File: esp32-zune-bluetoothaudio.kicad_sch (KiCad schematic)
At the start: 36 parts, among them J1 Conn_01x06, J2 USB_C_Receptacle_USB2.0, J3 zune connector, Q1 MMBT3904, Q2 MMBT3904, Q3 MMBT3904, Q4 MMBT3904, U1 TPM, U2 ESP32-A1S, U3 AP1117-33

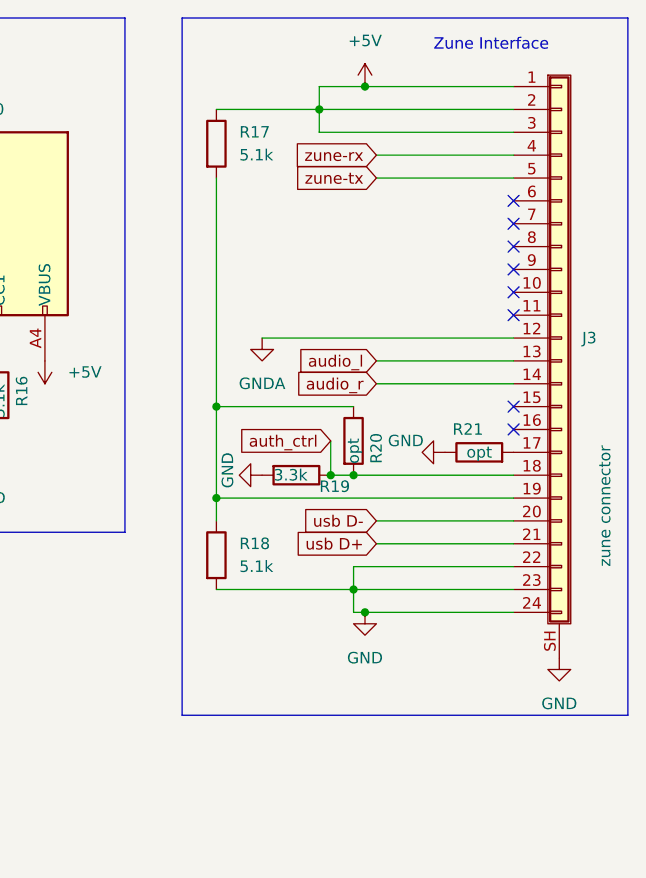
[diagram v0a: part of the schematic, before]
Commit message: layoutish
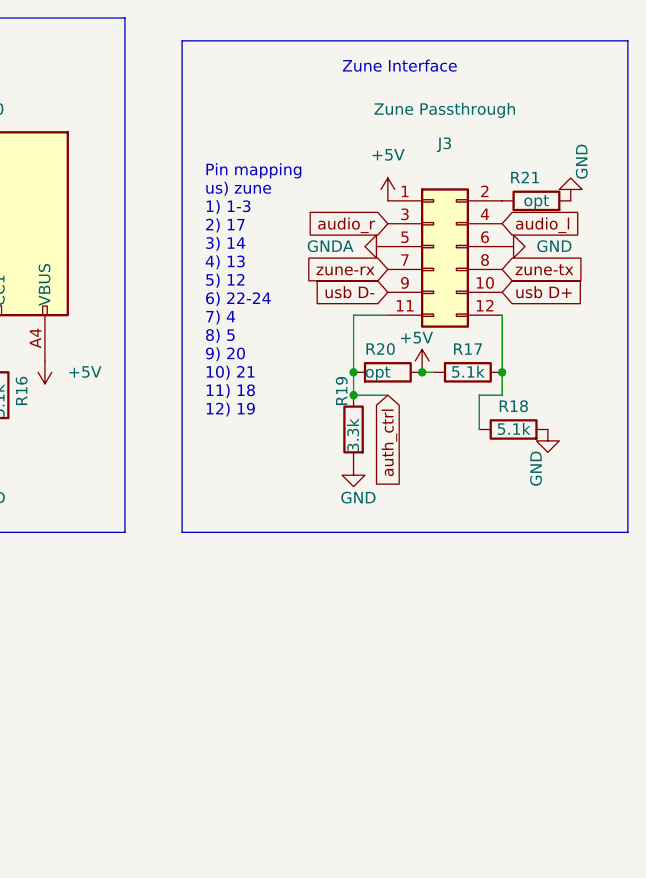
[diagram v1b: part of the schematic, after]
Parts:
- removed J3: zune connector, ZuneConnector:zune-edge-connector, symbol Connector_Generic_Shielded:Conn_01x24_Shielded
- added J3: Zune Passthrough, Connector_PinHeader_2.00mm:PinHeader_2x06_P2.00mm_Vertical_SMD, symbol Connector_Generic:Conn_02x06_Odd_Even
- J1: footprint Connector_PinSocket_2.54mm:PinSocket_1x06_P2.54mm_Horizontal -> Connector_PinHeader_2.54mm:PinHeader_1x06_P2.54mm_Vertical
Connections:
- net +5V: now also R17.2, R20.1, J3.1 (Pin_1); no longer R17.1
- net GND: now also R21.2, J3.6 (Pin_6); no longer R21.1
- net GNDA: now also J3.5 (Pin_5)
- net audio_l: now also J3.4 (Pin_4)
- net audio_r: now also J3.3 (Pin_3)
- net auth_ctrl: now also J3.11 (Pin_11)
- net usb D+: now also J3.10 (Pin_10)
- net usb D-: now also J3.9 (Pin_9)
- net zune-rx: now also J3.7 (Pin_7)
- net zune-tx: now also J3.8 (Pin_8)
- new net: J3.12 (Pin_12), R17.1, R18.1
- new net: J3.2 (Pin_2), R21.1
- no-connect marks 29 -> 21
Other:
- note added: "Pin mapping us) zune 1) 1-3 2) 17 3) 14 4) 13 5) 12 6) 22-24 7) 4 8) 5 9) 20 10) 21 11) 18 12) 19"
- moved on the sheet: R17, R18, R19, R20, R21
